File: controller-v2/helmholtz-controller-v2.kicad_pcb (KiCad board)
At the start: 2 copper layers, 36 parts, among them J1 Screw_Terminal_01x02, J2 Screw_Terminal_01x02, J3 Screw_Terminal_01x02, J4 Screw_Terminal_01x02, U1 BDS63150AFM, U2 BDS63150AFM, U3 INA226, U4 INA226, U5 BDS63150AFM, U6 INA226, U7 RPi_Pico

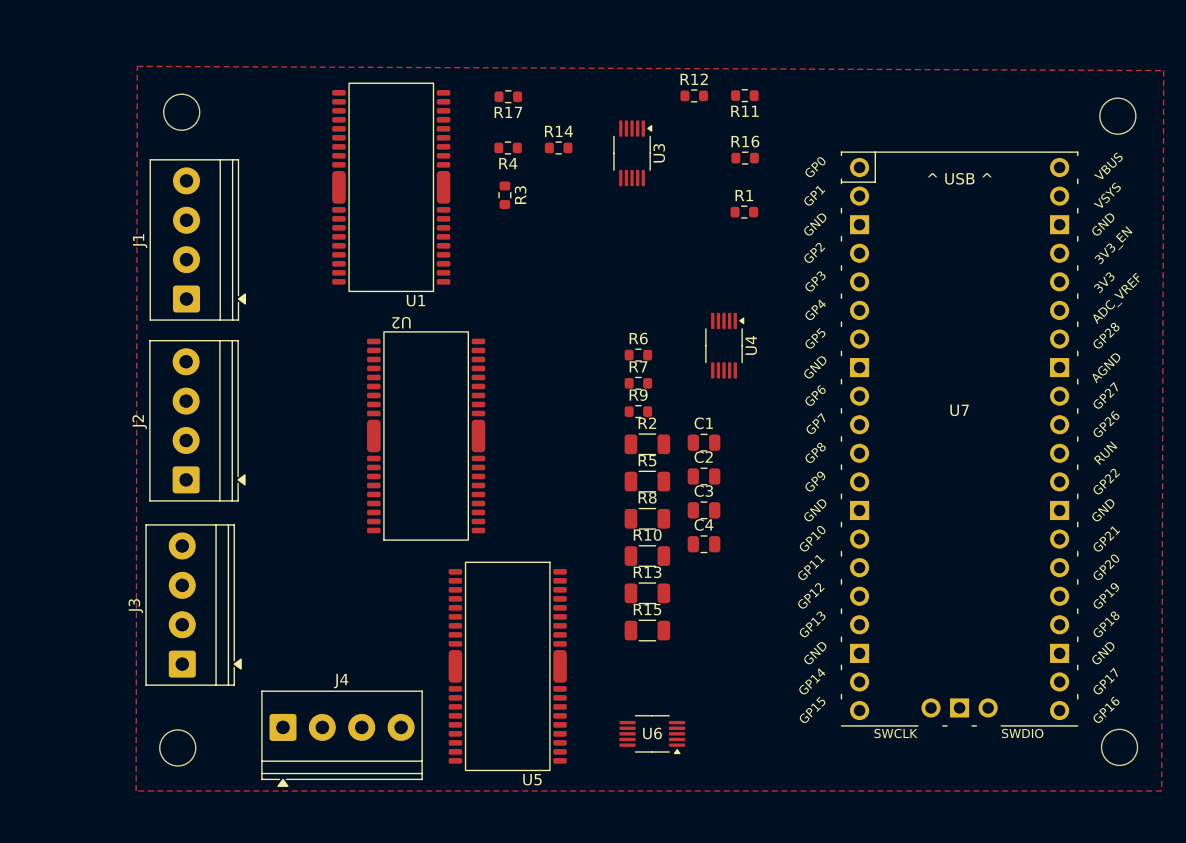
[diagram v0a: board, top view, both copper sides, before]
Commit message: Updated schematic & board
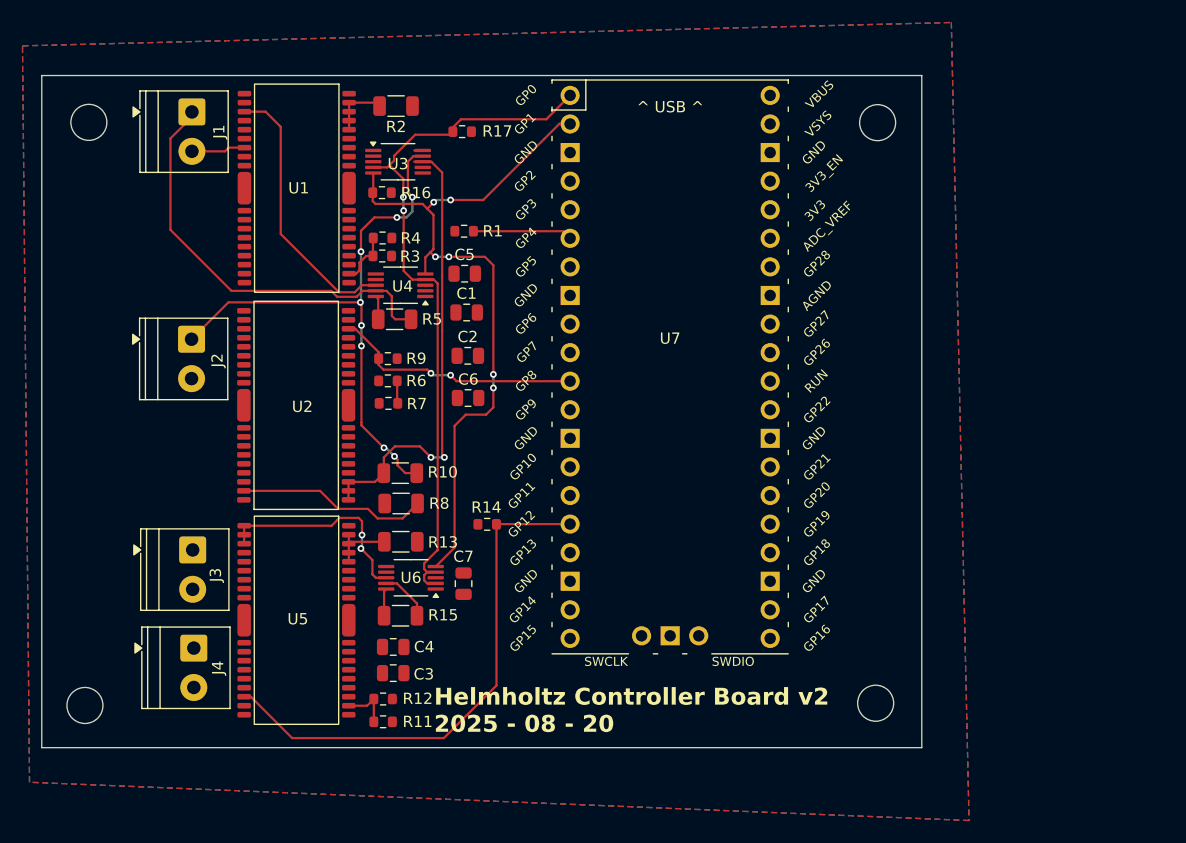
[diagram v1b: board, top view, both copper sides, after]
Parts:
- removed the REF** at (161.2, 55.1)
- removed the REF** at (77.6, 111.2)
- removed the REF** at (161.3, 111.2)
- removed the REF** at (78.0, 54.8)
- added C5: 1uF, Capacitor_SMD:C_0805_2012Metric, F.Cu at (103.1, 69.1)
- added C6: 1uF, Capacitor_SMD:C_0805_2012Metric, F.Cu at (103.4, 80.2)
- added C7: 1uF, Capacitor_SMD:C_0805_2012Metric, F.Cu at (103.0, 96.7)
- added REF**: MountingHole_3.2mm_M3, MountingHole:MountingHole_3.2mm_M3, F.Cu at (139.7, 107.3)
- added REF**: MountingHole_3.2mm_M3, MountingHole:MountingHole_3.2mm_M3, F.Cu at (69.7, 55.6)
- added REF**: MountingHole_3.2mm_M3, MountingHole:MountingHole_3.2mm_M3, F.Cu at (69.4, 107.5)
- added REF**: MountingHole_3.2mm_M3, MountingHole:MountingHole_3.2mm_M3, F.Cu at (139.8, 55.7)
- J1, J2, J3, J4: footprint TerminalBlock_Phoenix:TerminalBlock_Phoenix_PT-1,5-4-3.5-H_1x04_P3.50mm_Horizontal -> TerminalBlock_Phoenix:TerminalBlock_Phoenix_PT-1,5-2-3.5-H_1x02_P3.50mm_Horizontal
- R10, R13, R15, R2, R5, R8: value 0.1Ω -> 100m
- moved R11 64.3 mm to (95.9, 108.9)
- moved R12 60.3 mm to (95.9, 106.9), turned to 180 degrees
- moved R2 37.5 mm to (97.0, 54.2)
- moved R14 34.0 mm to (105.1, 91.4), turned to 180 degrees
- moved R16 32.4 mm to (95.8, 61.9)
- moved C3 31.2 mm to (96.8, 104.6)
- moved U4 29.2 mm to (97.4, 70.1), turned to 180 degrees
- moved C4 29.1 mm to (96.8, 102.3)
- moved R5 26.7 mm to (96.9, 73.2)
- moved U7 26.5 mm to (121.4, 77.4)
- moved U6 25.5 mm to (98.3, 96.1)
- moved R1 25.0 mm to (103.1, 65.3)
- moved C1 24.1 mm to (103.3, 72.5)
- moved C2 23.6 mm to (103.4, 76.4)
- moved R10 23.2 mm to (97.4, 86.8)
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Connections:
- R1 pad 1: Net-(U1-~{FAILA}) -> +3.3V
- R1 pad 2: +3.3V -> Net-(U1-~{FAILA})
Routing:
- net SCL: track 0.00 -> 65.8 mm, vias 0 -> 6
- net SDA: track 0.00 -> 63.0 mm, vias 0 -> 2
- net Net-(J2-Pin_1): track 0.00 -> 52.1 mm, vias 0 -> 8
- net Net-(U5-~{FAILA}): track 0.00 -> 46.8 mm
- net Net-(U3-Vbus): track 0.00 -> 41.7 mm, vias 0 -> 2
- net Net-(J1-Pin_1): track 0.00 -> 37.4 mm
- net Net-(U4-Vbus): track 0.00 -> 26.3 mm
- net Net-(U2-~{FAILA}): track 0.00 -> 22.3 mm, vias 0 -> 2
- net Net-(U6-Vbus): track 0.00 -> 21.5 mm, vias 0 -> 2
- net Net-(U2-RNFS): track 0.00 -> 17.0 mm
- net Net-(U1-~{FAILA}): track 0.00 -> 8.86 mm
- net Net-(U5-RNFS): track 0.00 -> 5.63 mm
- net Net-(U1-RNFS): track 0.00 -> 5.24 mm
- net Net-(J1-Pin_2): track 0.00 -> 4.80 mm
- net Net-(U1-VREF): track 0.00 -> 4.78 mm
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- added copper zone on B.Cu, net GND
- added copper zone on F.Cu, net GND
- removed copper zone on F.Cu, net (none)
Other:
- board outline added: 78.2 x 59.7 mm
- board text added: "Helmholtz Controller Board v2 2025 - 08 - 20"
